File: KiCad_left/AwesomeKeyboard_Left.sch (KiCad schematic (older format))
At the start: 57 parts, among them J1 AudioJack4_Ground, SW1 SW_DIP_x01, SW11 SW_Push, SW12 SW_Push, SW13 SW_Push, SW14 SW_Push, SW15 SW_Push, SW16 SW_Push, SW21 SW_Push, SW22 SW_Push, SW23 SW_Push, SW24 SW_Push, SW25 SW_Push, SW26 SW_Push, SW31 SW_Push, SW32 SW_Push, SW33 SW_Push, SW34 SW_Push, SW35 SW_Push, SW36 SW_Push, SW45 SW_Push, SW46 SW_Push

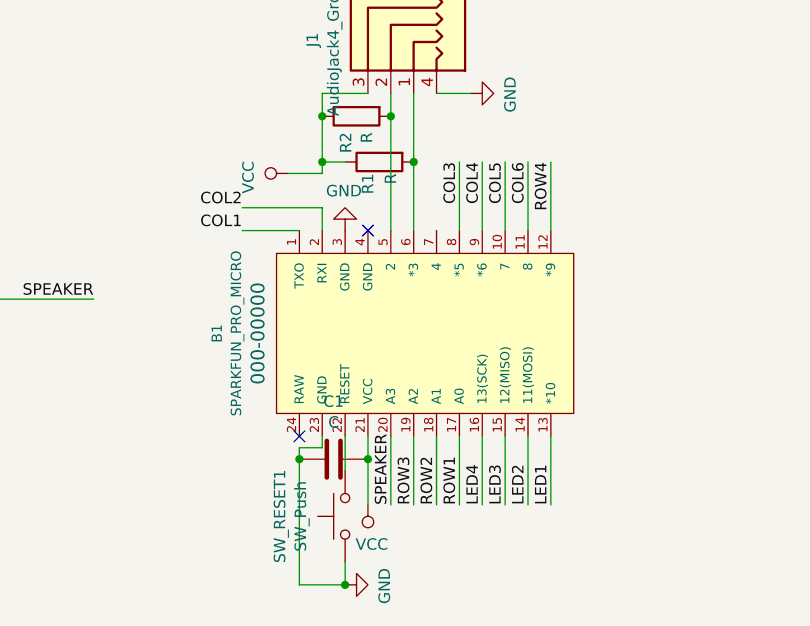
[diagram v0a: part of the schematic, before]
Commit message: re
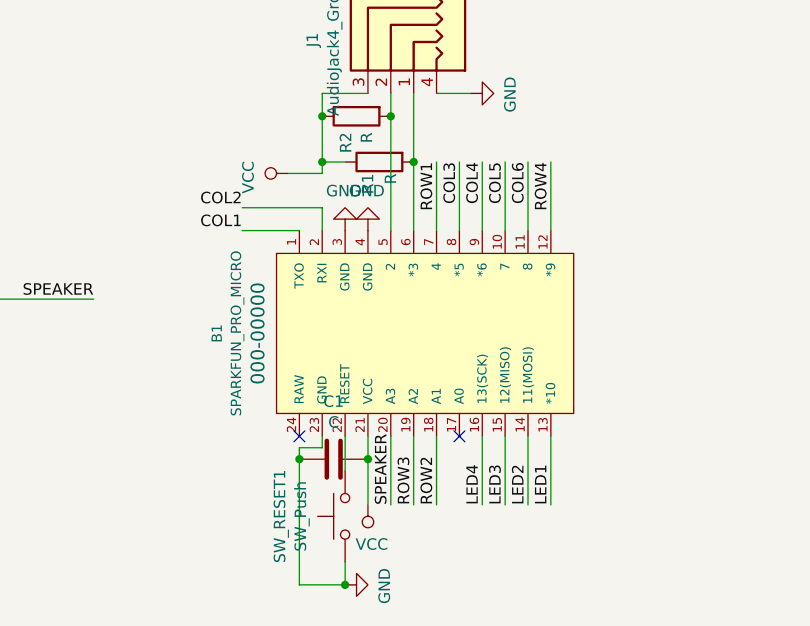
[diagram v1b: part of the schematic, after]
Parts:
- C1: footprint Capacitor_THT:CP_Axial_L10.0mm_D4.5mm_P15.00mm_Horizontal -> Capacitor_THT:CP_Radial_D4.0mm_P1.50mm
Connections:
- net GND: now also B1.4 (GND)
- net ROW1: now also B1.7 (4); no longer B1.17 (A0)
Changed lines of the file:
@@
 Wire Wire Line
 	5350 5650 5350 5350
-Text Label 5050 6850 1    50   ~ 0
+Text Label 4950 5350 3    50   ~ 0
 ROW1
 Text Label 4950 6850 1    50   ~ 0
@@
 ROW3
 Wire Wire Line
-	5050 6550 5050 6850
+	4950 5650 4950 5350
 Wire Wire Line
 	4950 6550 4950 6850
@@
 Text Label 5350 5350 3    50   ~ 0
 COL6
-NoConn ~ 4650 5650
 Wire Wire Line
 	4750 6550 4750 6850
@@
 F 0 "C1" V 4248 6650 50  0000 C CNN
 F 1 "C" V 4339 6650 50  0000 C CNN
-F 2 "Capacitor_THT:CP_Axial_L10.0mm_D4.5mm_P15.00mm_Horizontal" H 4538 6500 50  0001 C CNN
+F 2 "Capacitor_THT:CP_Radial_D4.0mm_P1.50mm" H 4538 6500 50  0001 C CNN
 F 3 "~" H 4500 6650 50  0001 C CNN
 	1    4500 6650
@@
 Wire Wire Line
 	4450 6600 4450 6550
+NoConn ~ 5050 6550
+$Comp
+L power:GND #PWR0113
+U 1 1 5C421C8C
+P 4650 5650
+F 0 "#PWR0113" H 4650 5400 50  0001 C CNN
+F 1 "GND" H 4655 5477 50  0000 C CNN
+F 2 "" H 4650 5650 50  0001 C CNN
+F 3 "" H 4650 5650 50  0001 C CNN
+	1    4650 5650
+	-1   0    0    1
+$EndComp
 $EndSCHEMATC
